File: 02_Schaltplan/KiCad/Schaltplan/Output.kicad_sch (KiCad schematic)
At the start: 22 parts, among them J10 Conn_02x01, J11 Conn_02x01, J12 Conn_02x01, J13 Conn_02x01, U23 74HC08PW

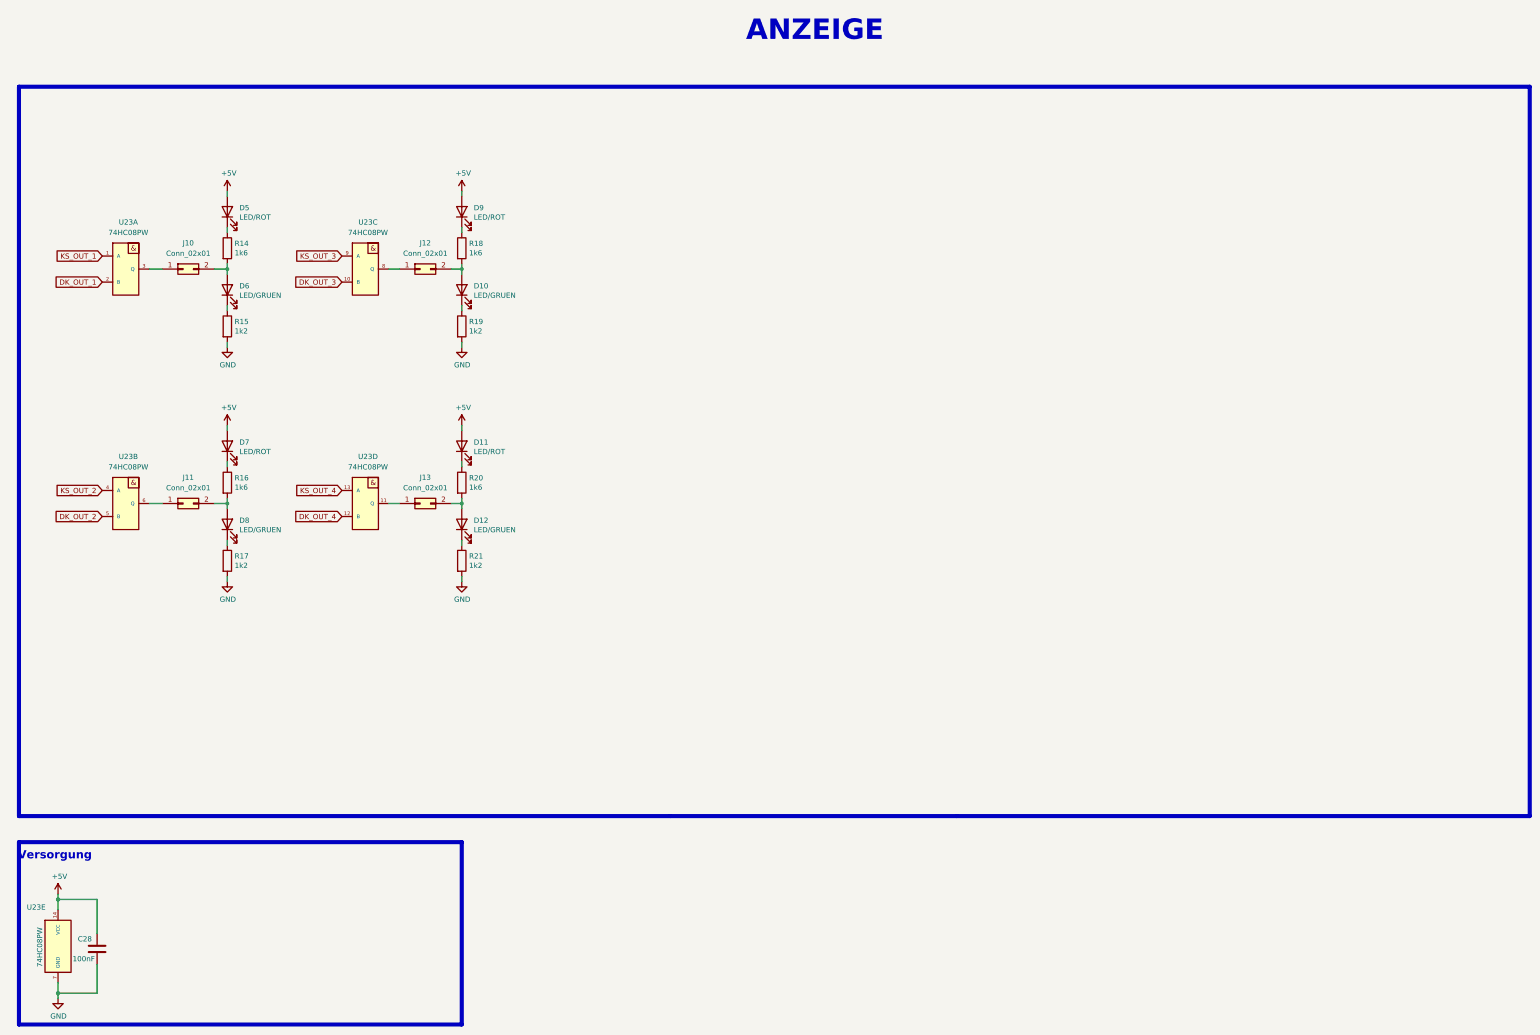
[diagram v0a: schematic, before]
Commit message: ADD
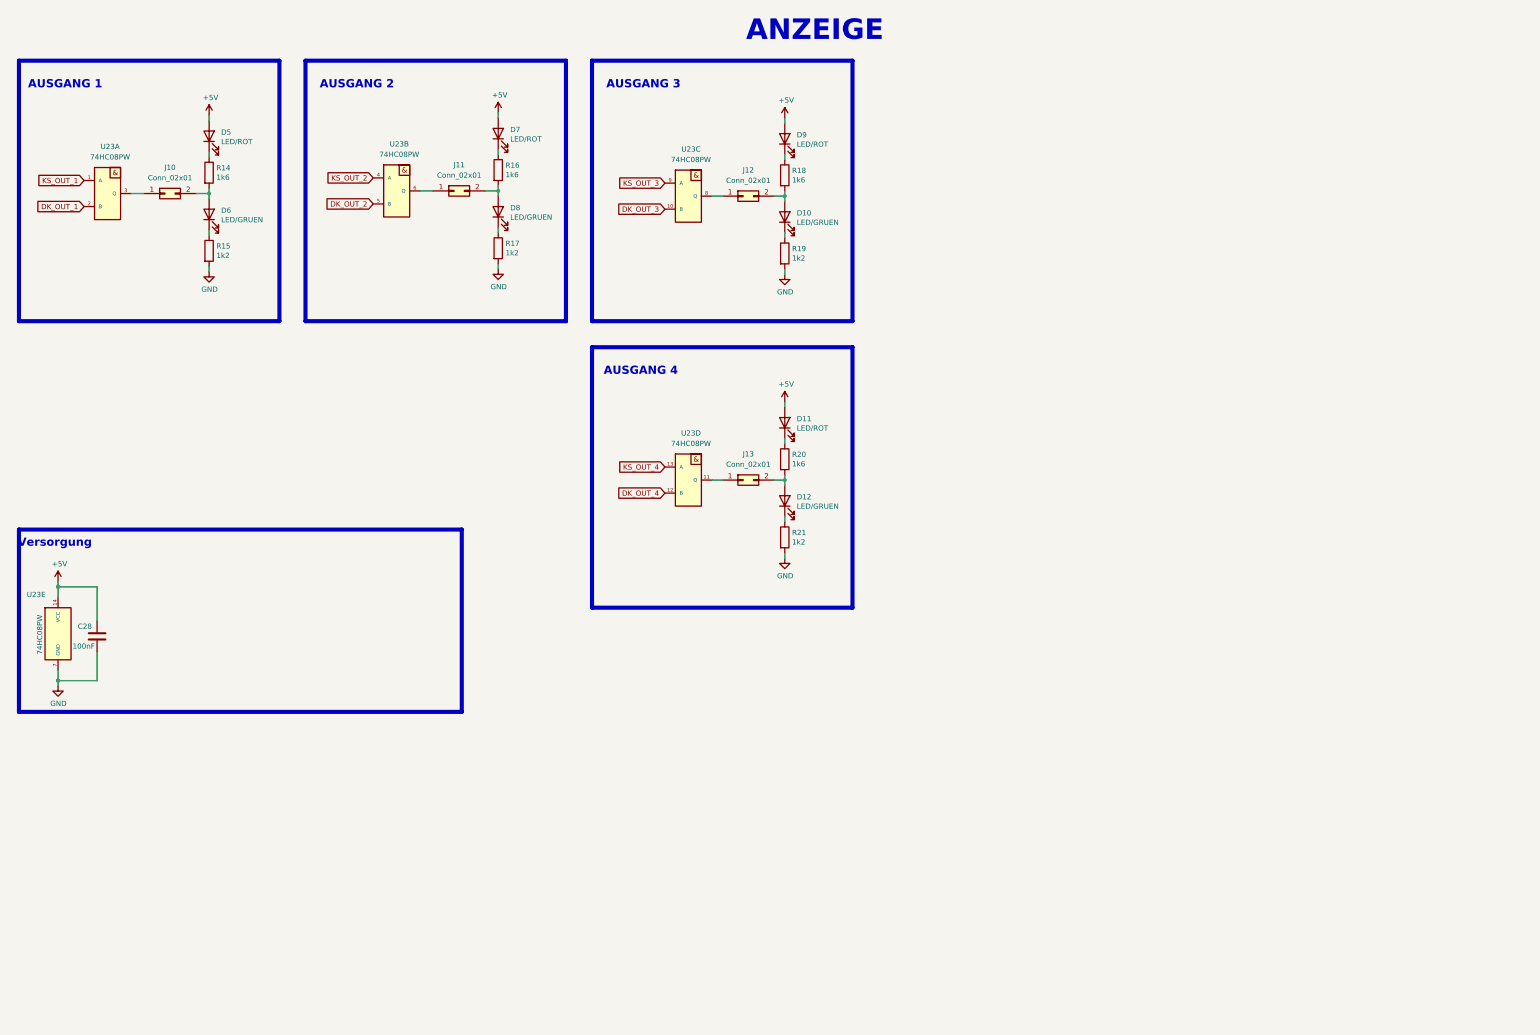
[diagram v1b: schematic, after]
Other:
- note added: "AUSGANG 1"
- note added: "AUSGANG 2"
- note added: "AUSGANG 3"
- note added: "AUSGANG 4"
- moved on the sheet: C28, D10, D11, D12, D5, D6, D7, D8, D9, J10, J11, J12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

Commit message: ADD
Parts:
- D10, D11, D12, D5, D6, D7, D8, D9: Stromaufnahme (none) -> 1mA
- U23: Stromaufnahme (none) -> 2uA
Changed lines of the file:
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@@
+      (effects (font (size 1.27 1.27)) hide)
+    )
+    (property "Stromaufnahme" "1mA" (id 4) (at 65.405 50.165 0)
       (effects (font (size 1.27 1.27)) hide)
     )
@@
       (effects (font (size 1.27 1.27)) hide)
     )
+    (property "Stromaufnahme" "1mA" (id 4) (at 65.405 69.215 0)
+      (effects (font (size 1.27 1.27)) hide)
+    )
     (pin "1")
     (pin "2")
@@
       (effects (font (size 1.27 1.27)) hide)
     )
+    (property "Stromaufnahme" "1mA" (id 4) (at 135.89 49.53 0)
+      (effects (font (size 1.27 1.27)) hide)
+    )
     (pin "1")
     (pin "2")
@@
       (effects (font (size 1.27 1.27)) hide)
     )
+    (property "Stromaufnahme" "1mA" (id 4) (at 135.89 68.58 0)
+      (effects (font (size 1.27 1.27)) hide)
+    )
     (pin "1")
     (pin "2")
@@
       (effects (font (size 1.27 1.27)) hide)
     )
+    (property "Stromaufnahme" "1mA" (id 4) (at 205.74 50.8 0)
+      (effects (font (size 1.27 1.27)) hide)
+    )
     (pin "1")
     (pin "2")
@@
       (effects (font (size 1.27 1.27)) hide)
     )
+    (property "Stromaufnahme" "1mA" (id 4) (at 205.74 69.85 0)
+      (effects (font (size 1.27 1.27)) hide)
+    )
     (pin "1")
     (pin "2")
@@
       (effects (font (size 1.27 1.27)) hide)
     )
+    (property "Stromaufnahme" "1mA" (id 4) (at 205.74 120.015 0)
+      (effects (font (size 1.27 1.27)) hide)
+    )
     (pin "1")
     (pin "2")
@@
     )
     (property "Mouser" "604-APT1608LZGCK" (id 4) (at 205.74 139.065 0)
+      (effects (font (size 1.27 1.27)) hide)
+    )
+    (property "Stromaufnahme" "1mA" (id 4) (at 205.74 139.065 0)
       (effects (font (size 1.27 1.27)) hide)
     )
@@
       (effects (font (size 1.27 1.27)) hide)
     )
+    (property "Stromaufnahme" "2uA" (id 4) (at 28.575 171.45 0)
+      (effects (font (size 1.27 1.27)) hide)
+    )
     (pin "14")
     (pin "7")
@@
       (effects (font (size 1.27 1.27)) hide)
     )
+    (property "Stromaufnahme" "2uA" (id 4) (at 40.64 64.135 0)
+      (effects (font (size 1.27 1.27)) hide)
+    )
     (pin "1")
     (pin "2")
@@
       (effects (font (size 1.27 1.27)) hide)
     )
+    (property "Stromaufnahme" "2uA" (id 4) (at 111.125 63.5 0)
+      (effects (font (size 1.27 1.27)) hide)
+    )
     (pin "4")
     (pin "5")
@@
       (effects (font (size 1.27 1.27)) hide)
     )
+    (property "Stromaufnahme" "2uA" (id 4) (at 182.245 64.77 0)
+      (effects (font (size 1.27 1.27)) hide)
+    )
     (pin "10")
     (pin "8")
@@
       (effects (font (size 1.27 1.27)) hide)
     )
+    (property "Stromaufnahme" "2uA" (id 4) (at 182.245 133.985 0)
+      (effects (font (size 1.27 1.27)) hide)
+    )
